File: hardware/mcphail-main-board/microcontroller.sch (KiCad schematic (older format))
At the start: 43 parts, among them J4 MICRO SD, J5 MICRO USB, J6 PROG/BOOT, J7 FONA 808, U5 ADS1118, U6 ATSAMD21G18A, U7 24AA1025 EEPROM, U8 MCP7940N RTC, X1 16MHz, X2 32.768kHz

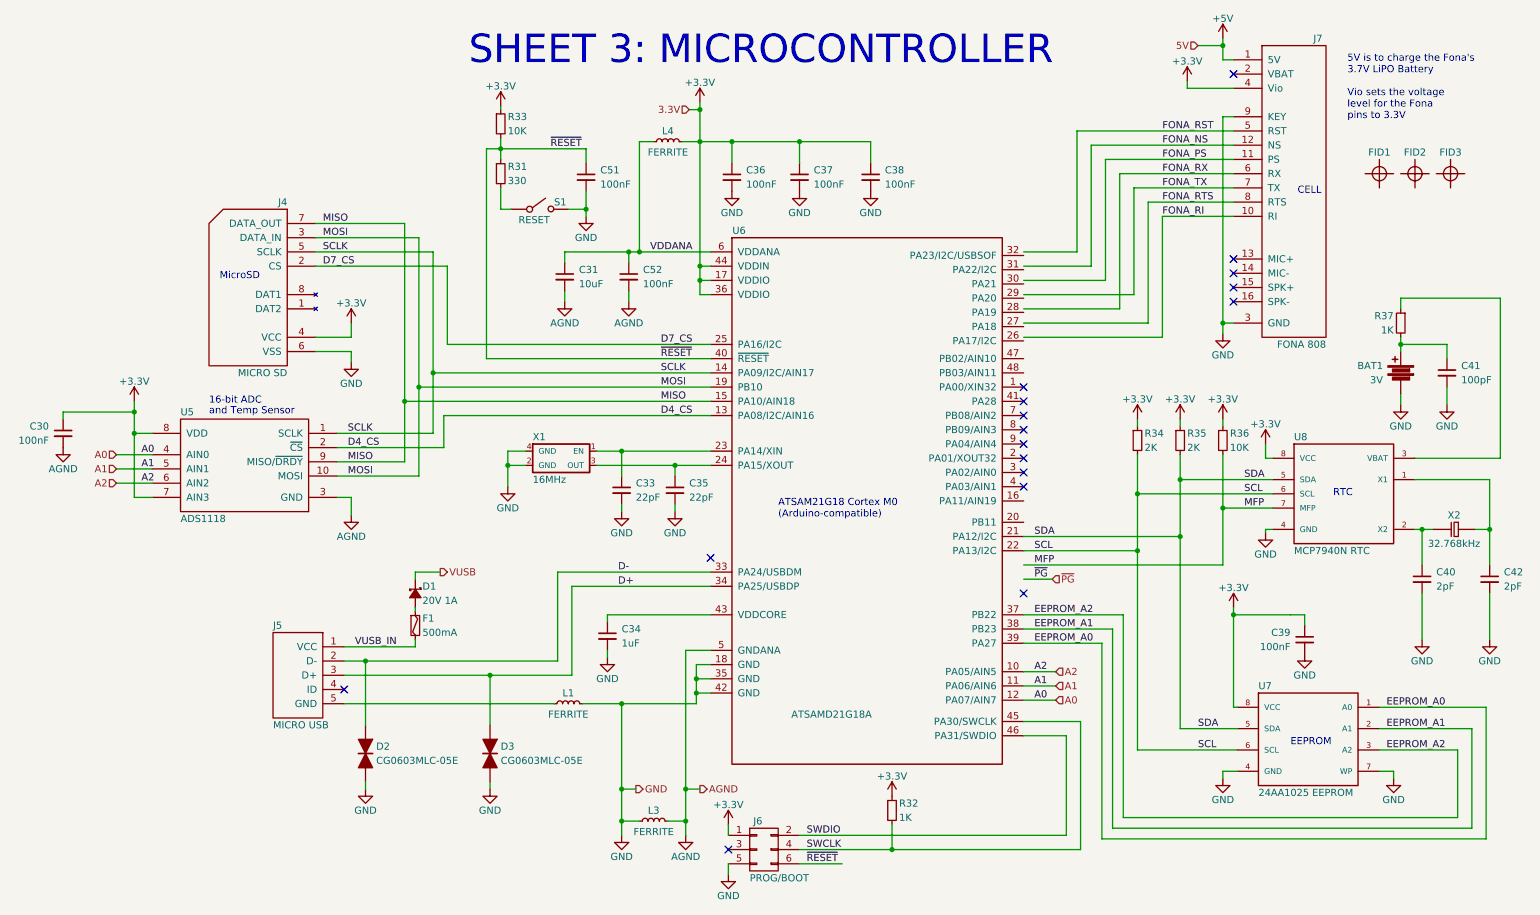
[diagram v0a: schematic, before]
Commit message: Regenerated sch pdf. Converted to 4 layer.
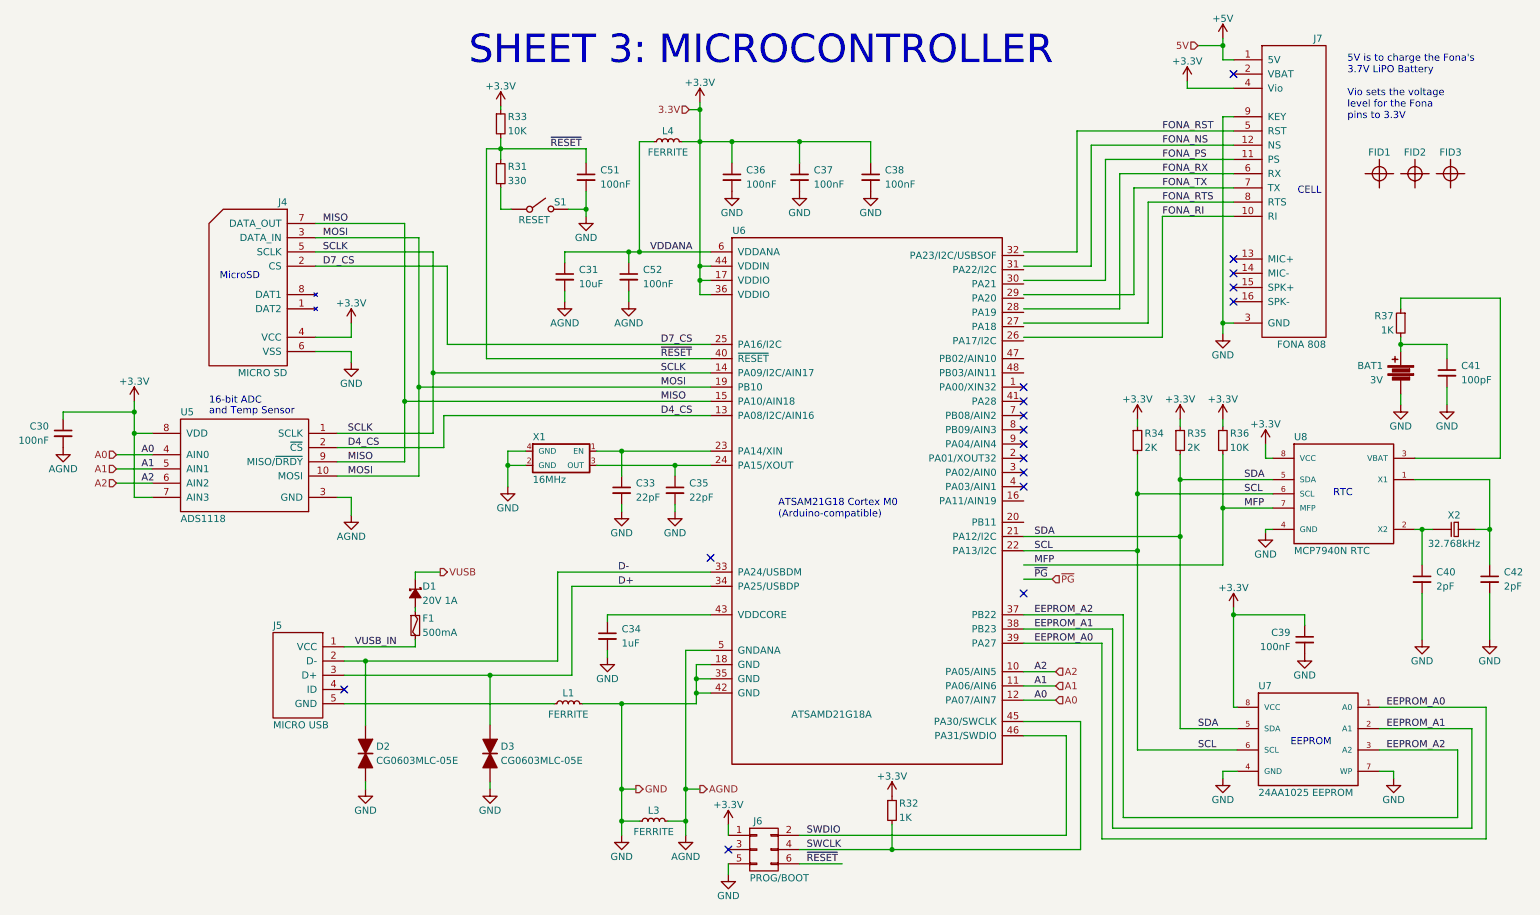
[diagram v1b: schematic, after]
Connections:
- wire segments 240 -> 198
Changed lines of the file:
@@
 SWCLK
 Wire Wire Line
-	3300 2025 3300 3275
-Wire Wire Line
-	3300 3275 3300 3700
+	3300 2025 3300 3700
 Wire Wire Line
 	7650 4875 8275 4875
@@
 Connection ~ 9050 2725
 Wire Wire Line
-	9050 1275 9050 2725
-Wire Wire Line
-	9050 2725 9050 2800
+	9050 1275 9050 2800
 Wire Wire Line
 	9050 2725 9125 2725
@@
 	8800 1075 9125 1075
 Wire Wire Line
-	9050 725  9050 775
-Wire Wire Line
-	9050 775  9050 875
+	9050 725  9050 875
 Wire Wire Line
 	9050 875  9125 875
@@
 Connection ~ 10450 4175
 Wire Wire Line
-	10925 3825 10925 4175
-Wire Wire Line
-	10925 4175 10925 4425
+	10925 3825 10925 4425
 Wire Wire Line
 	10450 4175 10450 4425
@@
 	10925 4625 10925 4950
 Wire Wire Line
-	10400 4175 10450 4175
-Wire Wire Line
-	10450 4175 10525 4175
+	10400 4175 10525 4175
 Wire Wire Line
 	10400 3825 10925 3825
 Connection ~ 8450 3925
 Wire Wire Line
-	8450 3650 8450 3925
-Wire Wire Line
-	8450 3925 8450 4325
-Wire Wire Line
-	8450 4325 8450 5725
+	8450 3650 8450 5725
 Connection ~ 8750 3825
 Wire Wire Line
-	8750 3650 8750 3825
-Wire Wire Line
-	8750 3825 8750 4225
-Wire Wire Line
-	8750 4225 8750 5575
+	8750 3650 8750 5575
 Connection ~ 9050 4025
 Wire Wire Line
-	9050 3650 9050 4025
-Wire Wire Line
-	9050 4025 9050 4425
+	9050 3650 9050 4425
 Wire Wire Line
 	11000 3675 10400 3675
@@
 	10300 3300 10300 3225
 Wire Wire Line
-	10300 2825 10300 2875
-Wire Wire Line
-	10300 2875 10300 2925
+	10300 2825 10300 2925
 Wire Wire Line
 	10150 5725 10700 5725
@@
 	9150 5875 9050 5875
 Wire Wire Line
-	9125 4725 9125 4775
-Wire Wire Line
-	9125 4775 9125 5425
+	9125 4725 9125 5425
 Wire Wire Line
 	9125 5425 9150 5425
@@
 	4575 1925 4450 1925
 Wire Wire Line
-	4575 1800 4575 1925
-Wire Wire Line
-	4575 1925 4575 1975
+	4575 1800 4575 1975
 Wire Wire Line
 	3975 1200 3975 1225
 Wire Wire Line
-	3400 2125 3400 3175
-Wire Wire Line
-	3400 3175 3400 3800
+	3400 2125 3400 3800
 Wire Wire Line
 	2675 2125 3400 2125
@@
 	3600 2875 3600 2325
 Wire Wire Line
-	3500 2225 3500 3075
-Wire Wire Line
-	3500 3075 3500 3500
+	3500 2225 3500 3500
 Wire Wire Line
 	2675 2225 3500 2225
@@
 	4150 3725 4025 3725
 Wire Wire Line
-	4025 3625 4025 3725
-Wire Wire Line
-	4025 3725 4025 3875
+	4025 3625 4025 3875
 Wire Wire Line
 	4150 3625 4025 3625
@@
 	5200 3800 5200 3725
 Wire Wire Line
-	4650 3725 5200 3725
-Wire Wire Line
-	5200 3725 5450 3725
-Wire Wire Line
-	4650 3625 4825 3625
-Wire Wire Line
-	4825 3625 5450 3625
+	4650 3725 5450 3725
+Wire Wire Line
+	4650 3625 5450 3625
 Wire Wire Line
 	3900 6000 3900 5950
@@
 	3025 5550 3025 5100
 Wire Wire Line
-	5350 5400 4825 5400
-Wire Wire Line
-	4825 5400 4550 5400
+	5350 5400 4550 5400
 Wire Wire Line
 	4375 5100 4375 4475
@@
 	4475 5200 4475 4575
 Wire Wire Line
-	2875 5200 3900 5200
-Wire Wire Line
-	3900 5200 4475 5200
-Wire Wire Line
-	2875 5100 3025 5100
-Wire Wire Line
-	3025 5100 4375 5100
+	2875 5200 4475 5200
+Wire Wire Line
+	2875 5100 4375 5100
 Wire Wire Line
 	2875 5400 4350 5400
@@
 	8625 2825 8625 1975
 Wire Wire Line
-	9125 4775 9525 4775
-Wire Wire Line
-	9525 4775 9625 4775
+	9125 4775 9625 4775
 Wire Wire Line
 	9625 4775 9625 4850
@@
 	1400 3500 1525 3500
 Wire Wire Line
-	1400 3275 1400 3350
-Wire Wire Line
-	1400 3350 1400 3500
-Wire Wire Line
-	1400 3500 1400 3950
+	1400 3275 1400 3950
 Wire Wire Line
 	1400 3950 1525 3950
@@
 	8800 1025 8800 1075
 Wire Wire Line
-	5375 1175 5375 1225
-Wire Wire Line
-	5375 1225 5375 1450
-Wire Wire Line
-	5375 1450 5375 2325
-Wire Wire Line
-	5375 2325 5375 2425
-Wire Wire Line
-	5375 2425 5375 2525
+	5375 1175 5375 2525
 Wire Wire Line
 	5450 4775 4725 4775
@@
 	5450 5125 5350 5125
 Wire Wire Line
-	5350 5125 5350 5225
-Wire Wire Line
-	5350 5225 5350 5325
-Wire Wire Line
-	5350 5325 5350 5400
+	5350 5125 5350 5400
 Wire Wire Line
 	5450 5325 5350 5325
@@
 Connection ~ 5350 5225
 Wire Wire Line
-	5275 5025 5275 6000
-Wire Wire Line
-	5275 6000 5275 6225
-Wire Wire Line
-	5275 6225 5275 6325
+	5275 5025 5275 6325
 Wire Wire Line
 	5275 5025 5450 5025
 Wire Wire Line
-	4825 5400 4825 6000
-Wire Wire Line
-	4825 6000 4825 6225
-Wire Wire Line
-	4825 6225 4825 6325
+	4825 5400 4825 6325
 Wire Wire Line
 	5275 6225 5150 6225
@@
 Connection ~ 4825 5400
 Wire Wire Line
-	4425 2225 4875 2225
-Wire Wire Line
-	4875 2225 4950 2225
-Wire Wire Line
-	4950 2225 5450 2225
+	4425 2225 5450 2225
 Wire Wire Line
 	4875 2225 4875 2300
@@
 Connection ~ 4950 2225
 Wire Wire Line
-	3975 1425 3975 1500
-Wire Wire Line
-	3975 1500 3975 1575
+	3975 1425 3975 1575
 Wire Wire Line
 	3975 1775 3975 1925
@@
 	4575 1500 4575 1600
 Wire Wire Line
-	3875 1500 3975 1500
-Wire Wire Line
-	3975 1500 4575 1500
+	3875 1500 4575 1500
 Connection ~ 3975 1500
 Wire Wire Line
@@
 	7950 5625 7650 5625
 Wire Wire Line
-	6075 6425 6725 6425
-Wire Wire Line
-	6725 6425 8050 6425
+	6075 6425 8050 6425
 Wire Wire Line
 	8050 6425 8050 5525
@@
 $EndComp
 Wire Wire Line
-	5250 1450 5375 1450
-Wire Wire Line
-	5375 1450 5600 1450
-Wire Wire Line
-	5600 1450 6075 1450
-Wire Wire Line
-	6075 1450 6575 1450
+	5250 1450 6575 1450
 $Comp
 L FIDUCIAL FID1
